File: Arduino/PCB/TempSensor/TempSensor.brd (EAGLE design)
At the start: 32.7 x 32.4 mm, 41 parts, among them IC1 DS1820, J1 FTDI_DEVICE, J2 FTDI_DEVICE, U1 ATMEGA328-AU, X1 16Mhz

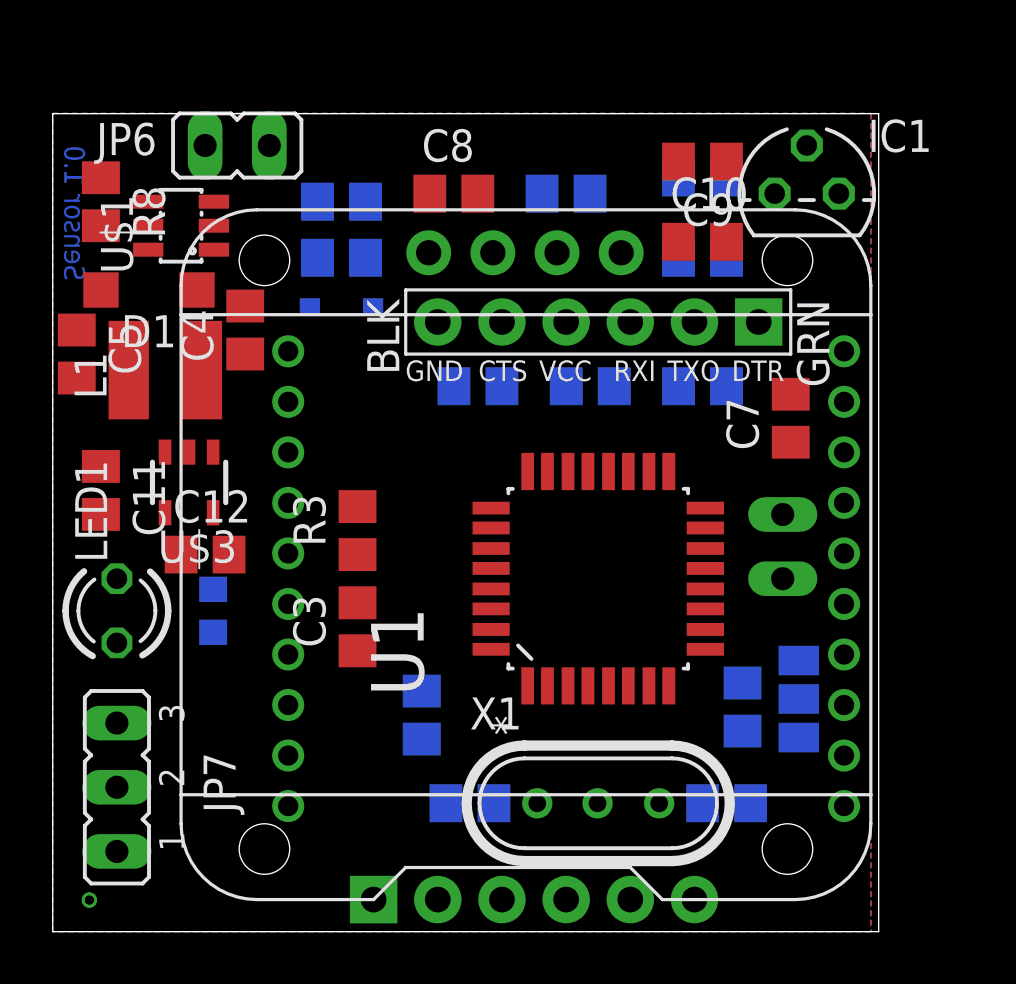
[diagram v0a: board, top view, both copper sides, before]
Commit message: met manuele routing power
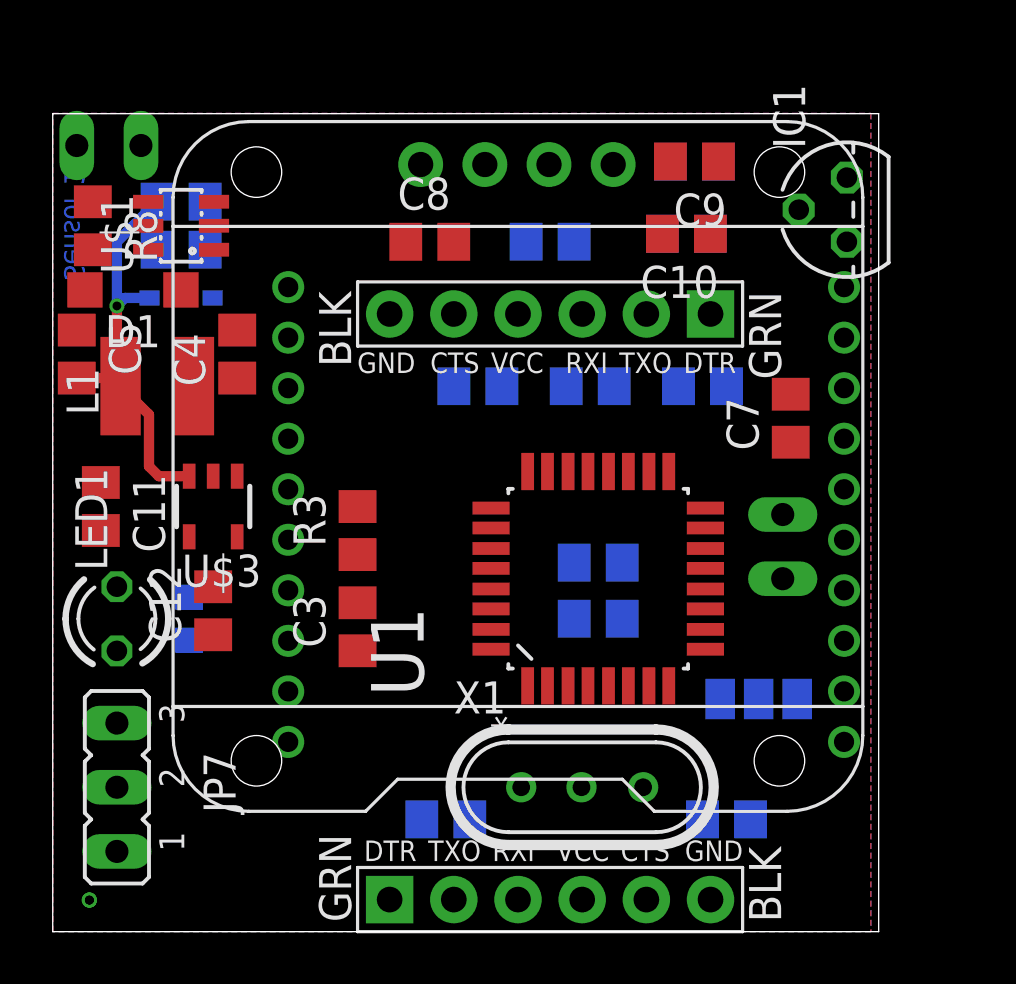
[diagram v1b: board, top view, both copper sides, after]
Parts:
- moved R7 8.08 mm to (58.4, 34.9), turned to 0 degrees
- moved R6 7.96 mm to (58.4, 32.7), turned to 0 degrees
- moved D2 6.36 mm to (41.9, 45.4), turned to 0 degrees
- moved R10 6.36 mm to (41.9, 47.3), turned to 180 degrees
- moved R9 6.35 mm to (41.9, 49.2), turned to 0 degrees
- moved JP6 5.08 mm to (39.1, 51.4), flipped to the bottom, turned to 270 degrees
- moved U$2 3.51 mm to (55.6, 39.1)
- moved XB1 2.54 mm to (57.1, 36.8)
- moved C12 2.25 mm to (43.2, 33.0), turned to 90 degrees
- moved C8 2.13 mm to (51.8, 47.6)
- moved R5 2.01 mm to (56.5, 47.6)
- moved J2 1.93 mm to (56.5, 44.8)
- moved IC1 1.71 mm to (68.3, 48.9), turned to 90 degrees
- moved SJ2 1.59 mm to (64.8, 29.5), turned to 180 degrees
- moved U$3 1.35 mm to (43.2, 37.1)
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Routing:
- net VO: track 0.00 -> 16.5 mm, vias 0 -> 1
